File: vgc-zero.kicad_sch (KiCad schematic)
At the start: 22 parts, among them J1 Conn_01x06_Pin, J2 Conn_01x06_Pin, J3 Conn_01x06_Pin, SW1 SW_Push, SW10 SW_Push, SW11 SW_SPDT, SW2 SW_Push, SW3 SW_Push, SW4 SW_Push, SW5 SW_Push, SW6 SW_Push, SW7 SW_Push, SW8 SW_Push, SW9 SW_Push

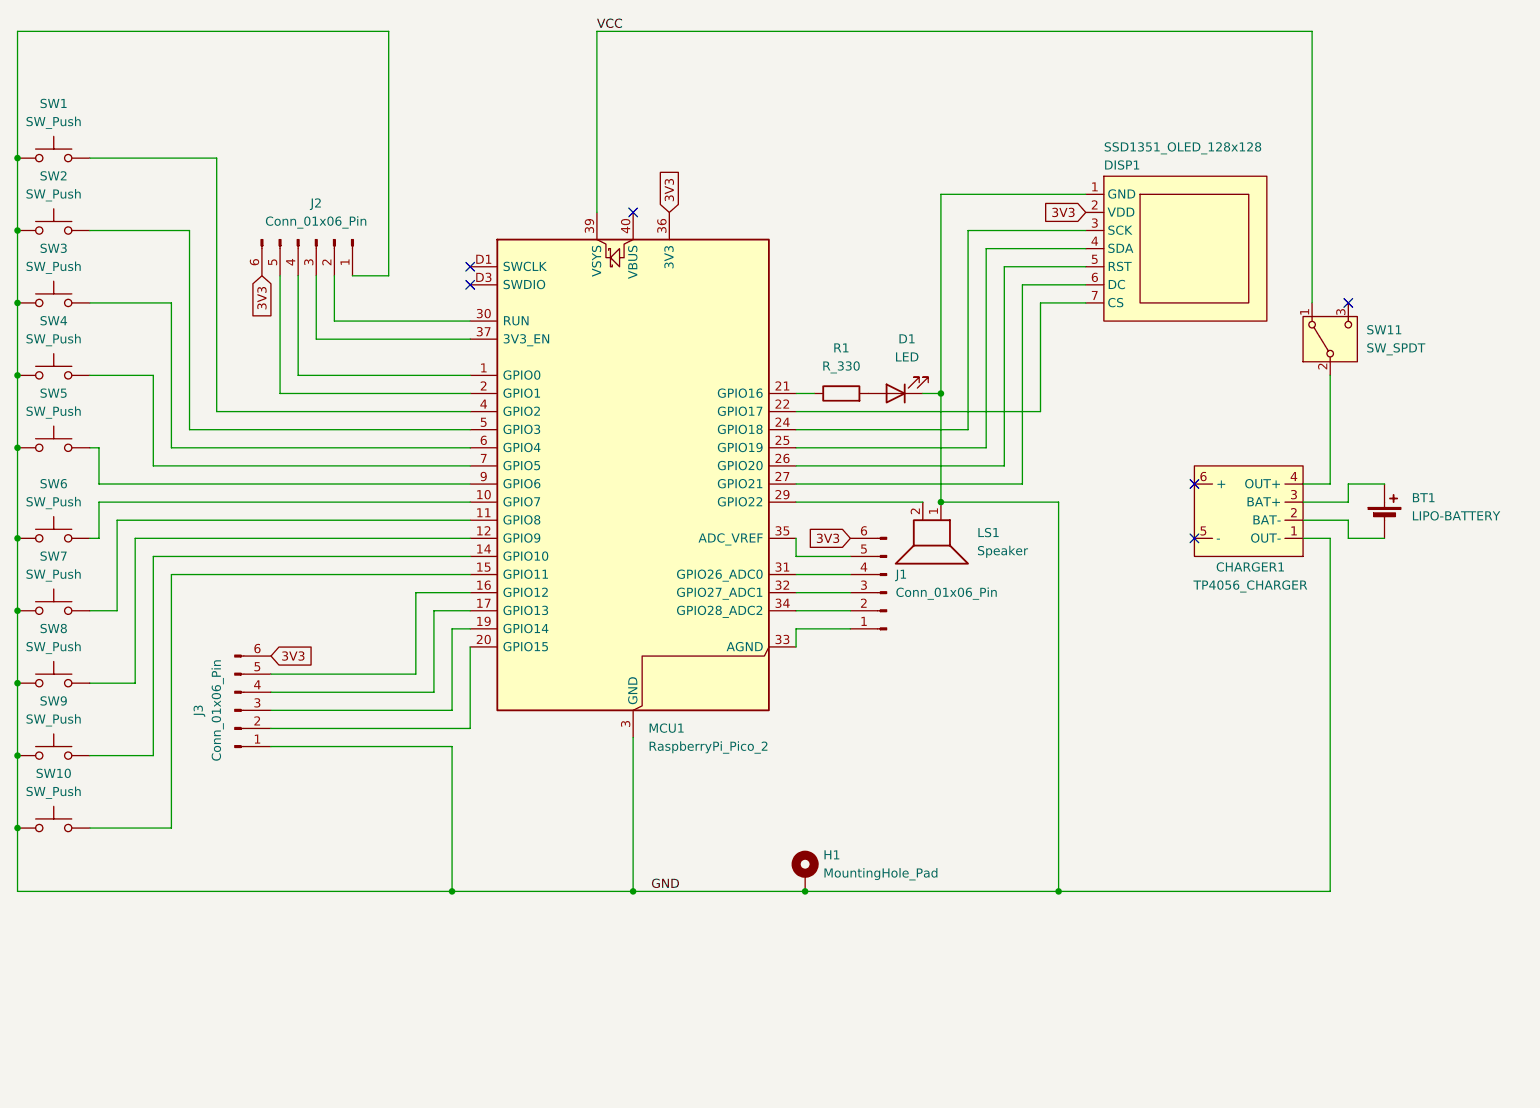
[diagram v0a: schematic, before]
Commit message: update to 1.1.0
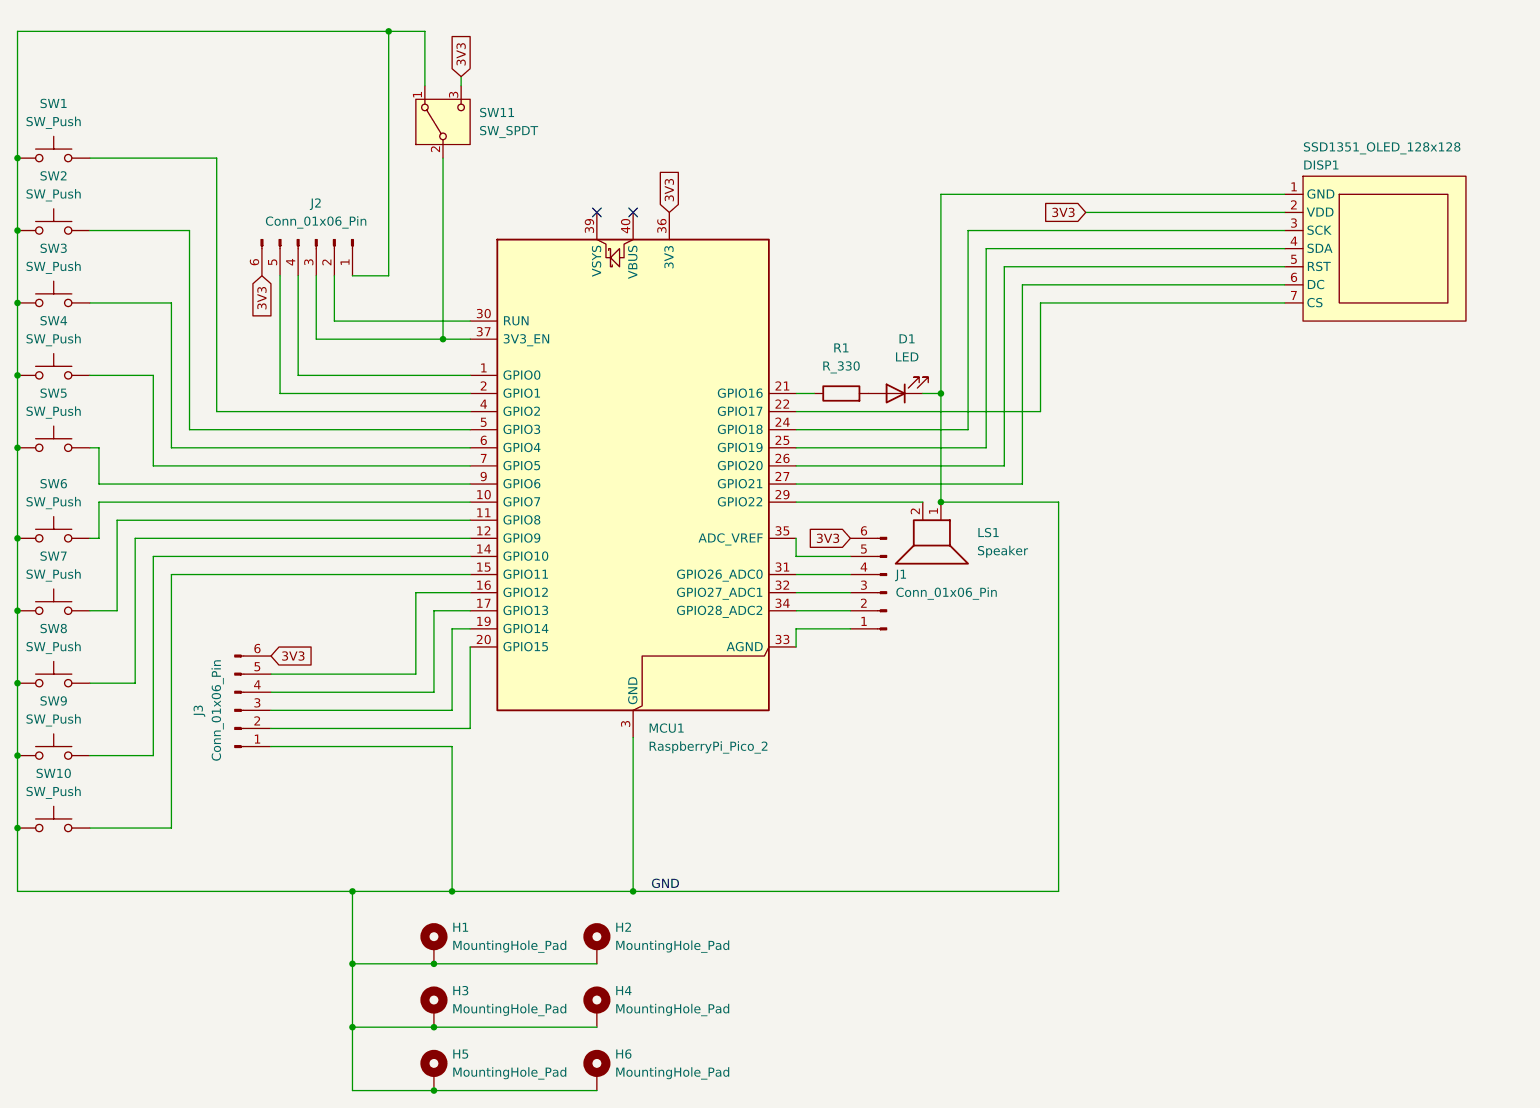
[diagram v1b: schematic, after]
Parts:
- removed BT1: LIPO-BATTERY, Connector_JST:JST_PH_S2B-PH-K_1x02_P2.00mm_Horizontal, symbol Device:Battery_Cell
- removed CHARGER1: TP4056_CHARGER, vgc-zero-footprints:Tp4056_Charger, symbol vgc-zero-symbols:TP4056_CHARGER
- added H2, H3, H4, H5, H6: MountingHole_Pad, MountingHole:MountingHole_2.2mm_M2_Pad, symbol Mechanical:MountingHole_Pad
- DISP1: footprint vgc-zero-footprints:SSD1351_OLED_128x128 -> Connector_JST:JST_PH_S7B-PH-K_1x07_P2.00mm_Horizontal
- H1: footprint MountingHole:MountingHole_3.2mm_M3_Pad -> MountingHole:MountingHole_2.2mm_M2_Pad
- LS1: footprint Connector_Wire:SolderWire-0.1sqmm_1x02_P3.6mm_D0.4mm_OD1mm -> Buzzer_Beeper:Buzzer_12x9.5RM7.6
- MCU1: footprint Module:RaspberryPi_Pico_SMD_HandSolder -> Module:RaspberryPi_Pico_Common_THT; symbol MCU_Module:RaspberryPi_Pico_Debug -> MCU_Module:RaspberryPi_Pico
- SW1, SW10, SW2, SW3, SW4, SW5, SW6, SW7, SW8, SW9: footprint vgc-zero-footprints:SW_PUSH_RUBBER_8mm -> Button_Switch_THT:SW_PUSH_6mm_H5mm
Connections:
- net 3V3: now also SW11.3 (C)
- net GND: now also SW11.1 (A), H2.1, H3.1, H4.1, H5.1, H6.1; no longer MCU1.D2 (GND)
- net at SW11.2 (B): now also J2.3 (Pin_3), MCU1.37 (3V3_EN)
- net VCC: no longer names the net of MCU1.39 (VSYS)
- net VCC: no longer SW11.1 (A)
- no-connect marks 6 -> 2
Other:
- moved on the sheet: DISP1, SW11
